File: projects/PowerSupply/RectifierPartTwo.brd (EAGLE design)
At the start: 90 x 65 mm, 13 parts, among them K1 G2R2, X1 LINE-IN, X2 T2-PRI, X3 T2-SEC, X4 R2-OUT

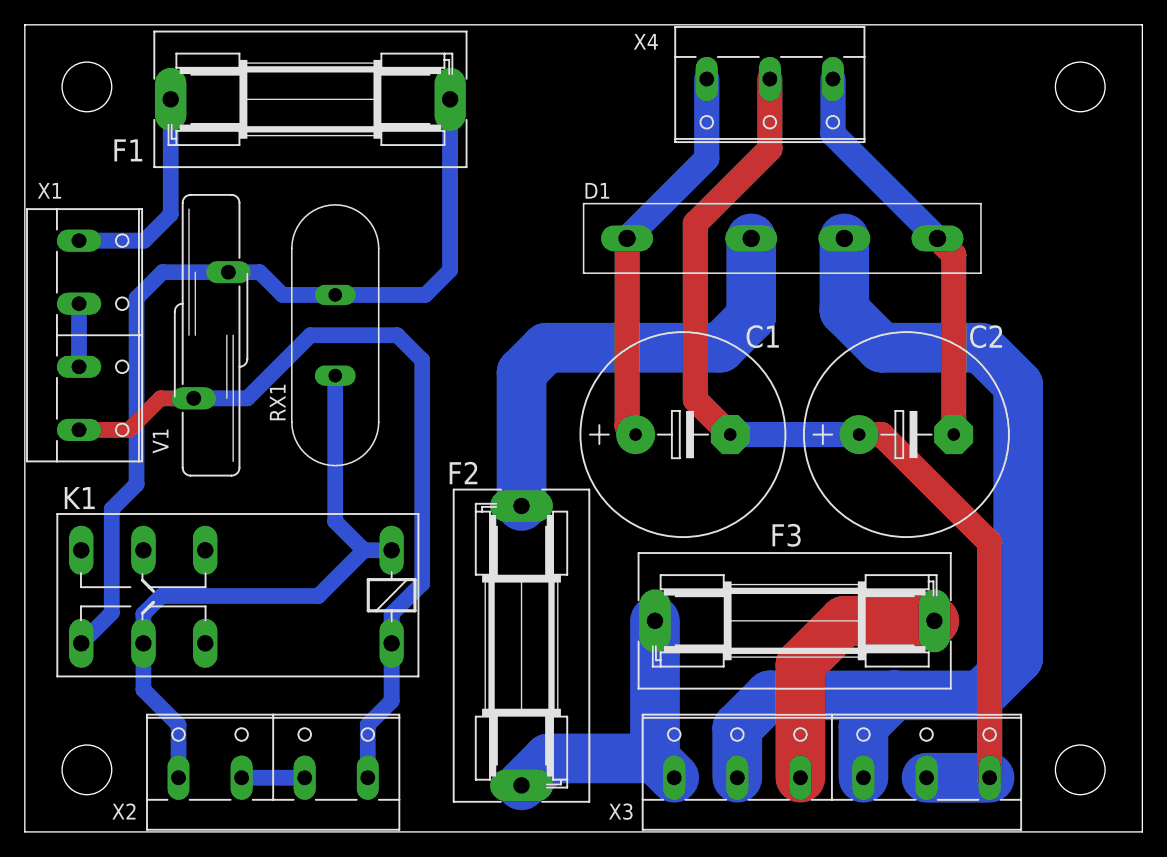
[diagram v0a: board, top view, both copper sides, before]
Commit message: feat: rectifier part two modified
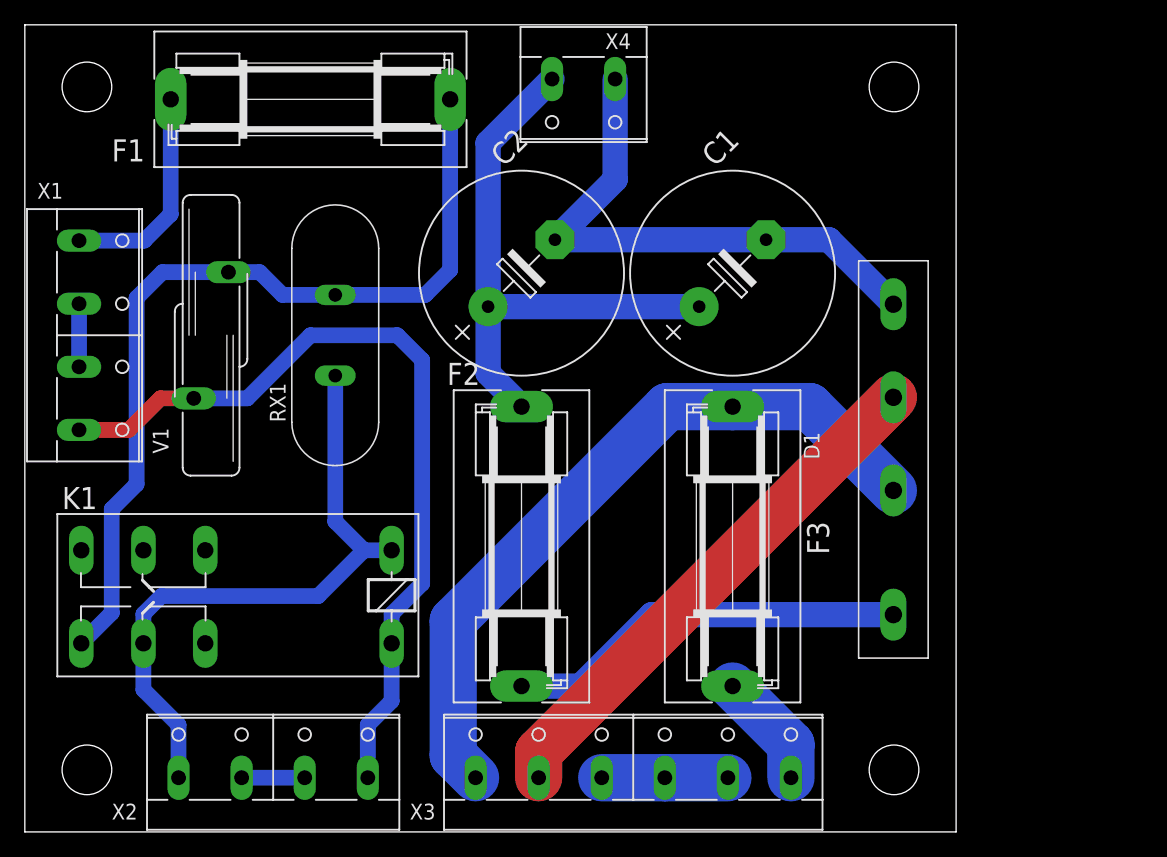
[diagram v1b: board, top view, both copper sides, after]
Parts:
- C2: value 2200µF -> 4700µF
- F2: value 6.3AT -> 4A
- X4: value R2-OUT -> (none); device con-wago-508:W237-133 -> con-wago-508:W237-132
- moved C2 33.6 mm to (40.0, 45.0), turned to 45 degrees
- moved D1 29.2 mm to (70.0, 30.0), turned to 90 degrees
- moved X3 16.0 mm to (49.0, 5.00)
- moved X4 15.0 mm to (45.0, 60.0)
- moved C1 13.6 mm to (57.0, 45.0), turned to 45 degrees
- moved F2 8.00 mm to (40.0, 23.0)
- moved F3 7.81 mm to (57.0, 23.0), turned to 90 degrees
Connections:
- removed net GND: C1.-, C2.+, X3.5, X3.6, X4.2
- removed net N$20: C1.+, D1.+VDC, X4.3
- removed net N$21: C2.-, D1.-VDC, X4.1
- new net N$1: D1.VAC2, X3.2
- new net N$4: F3.1, X3.6
- net N$2: now also D1.VAC1, F3.2, X3.1; no longer D1.VAC2, X3.2, X3.4
- net N$3: now also D1.+VDC; no longer F3.2, X3.1
- net N$5: now also C1.+, C2.+, X4.2; no longer D1.VAC1
- net N$6: now also C1.-, C2.-, D1.-VDC, X4.1; no longer F3.1, X3.3
- net PE: now also X3.3, X3.4, X3.5
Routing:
- net GND: track 80.8 -> 0.00 mm
- net N$1: track 0.00 -> 42.5 mm
- net N$21: track 32.7 -> 0.00 mm
- net N$20: track 31.6 -> 0.00 mm
- net N$6: track 21.4 -> 44.4 mm
- net N$2: track 80.9 -> 58.8 mm
- net PE: track 5.08 -> 15.2 mm
- net N$4: track 0.00 -> 9.33 mm
- net N$5: track 37.4 -> 46.6 mm
- net N$3: track 24.9 -> 32.3 mm
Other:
- board size 90 x 65 mm -> 75 x 65 mm
